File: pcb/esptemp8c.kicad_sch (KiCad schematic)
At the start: 19 parts, among them J1 T1, J2 T2, J4 T3, J6 T4, SW1 RESET, U1 ESP32-C3-MINI-1

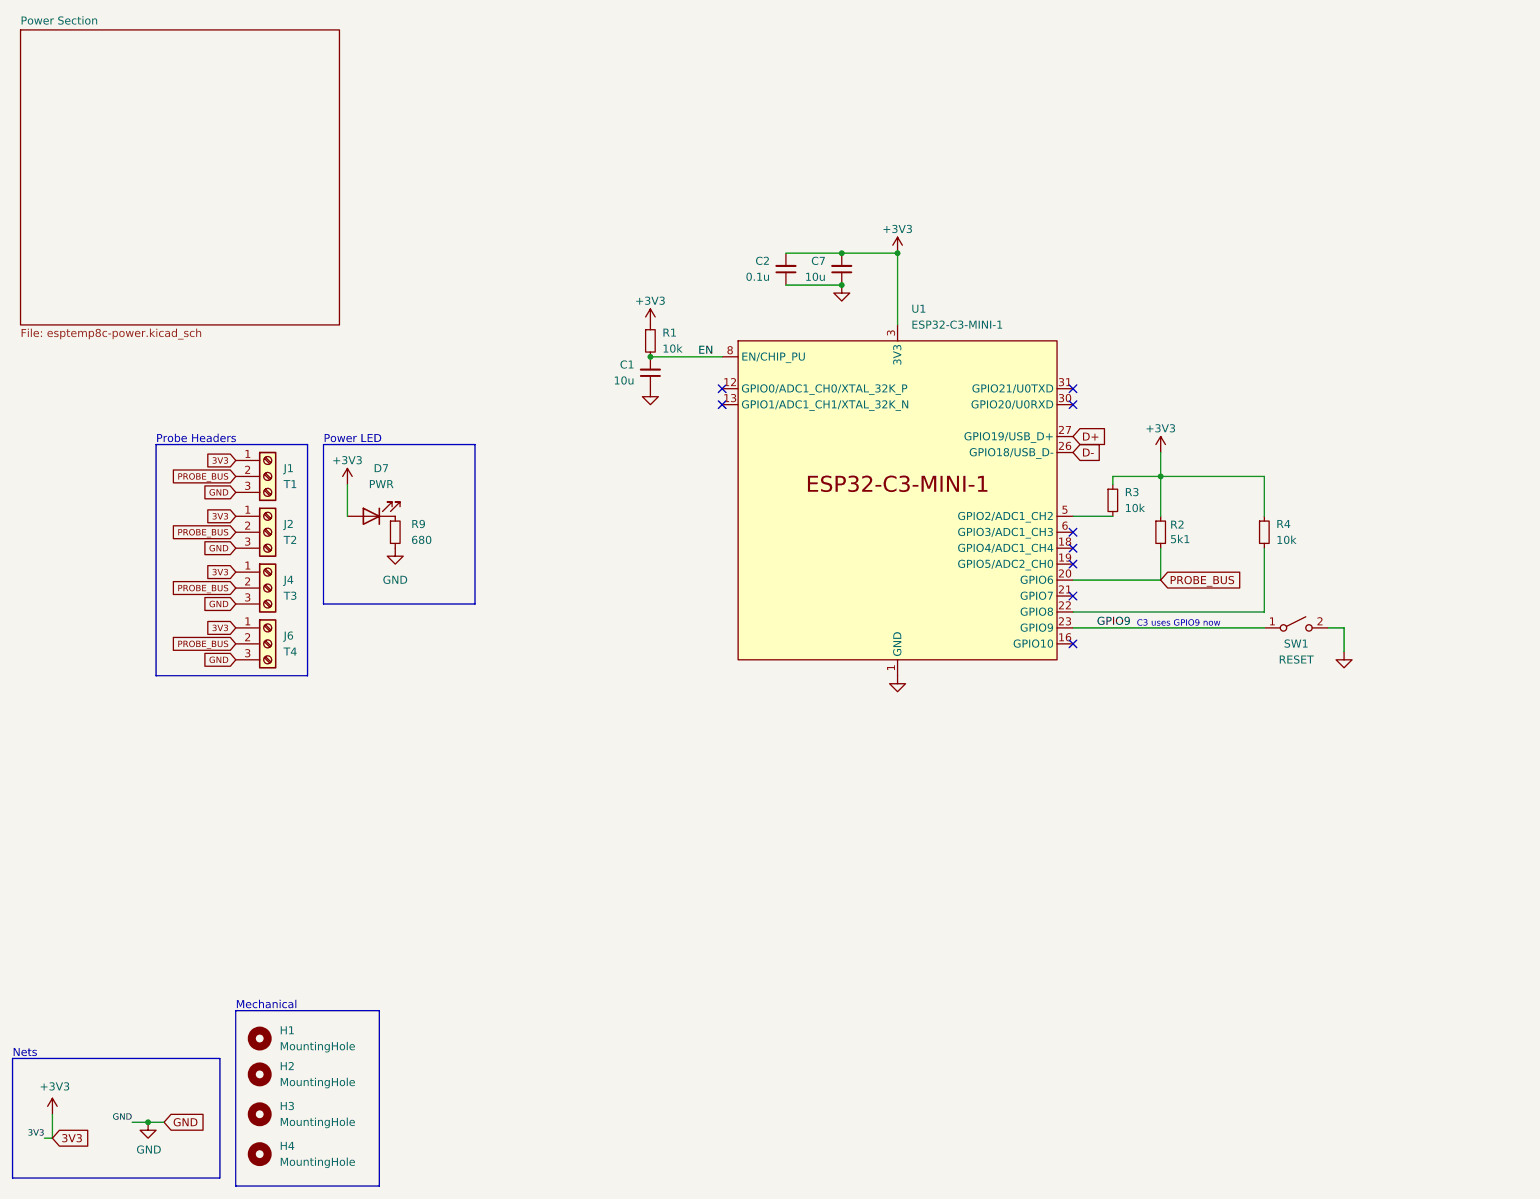
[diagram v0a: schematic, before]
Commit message: final touches and check
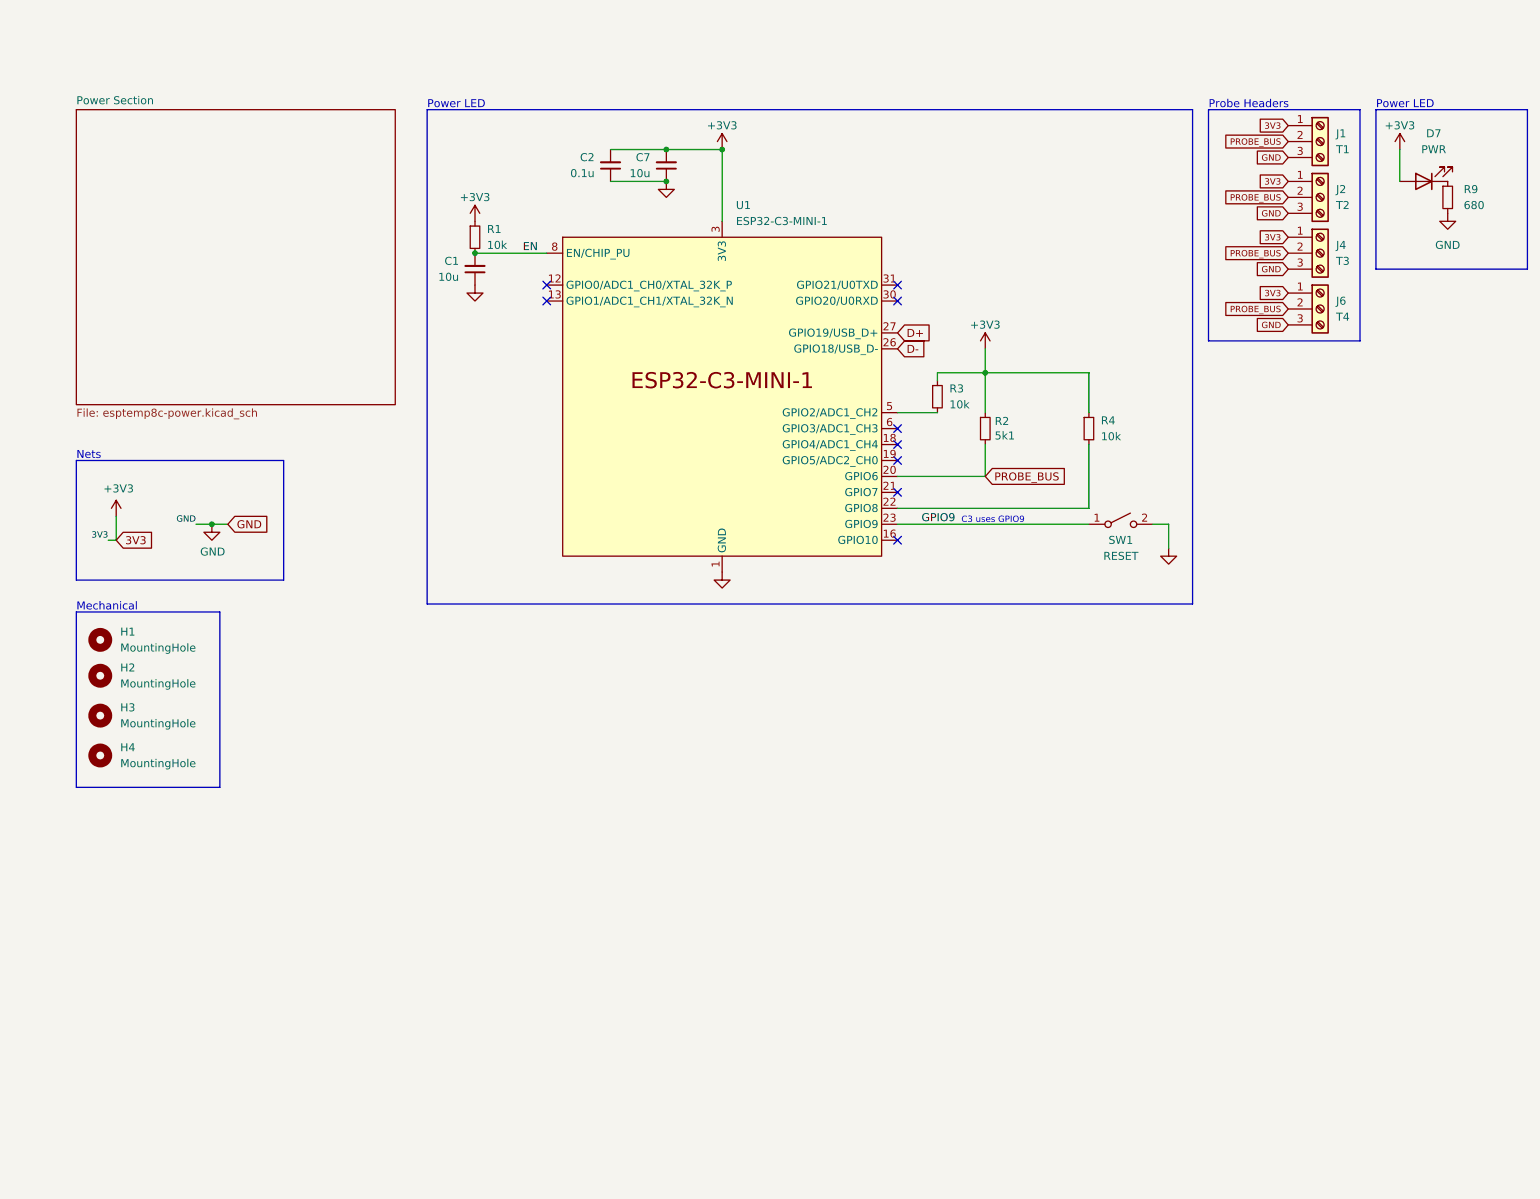
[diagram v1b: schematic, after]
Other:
- note added: "C3 uses GPIO9"
- note removed: "C3 uses GPIO9 now"
- moved on the sheet: C1, C2, C7, D7, H1, H2, H3, H4, J1, J2, J4, J6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

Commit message: panel touchup, alternate pn
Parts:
- J1, J2, J6: LCSC Alt (none) -> C5188158
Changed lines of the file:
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@@
+			)
+		)
+		(property "LCSC Alt" "C5188158"
+			(at 222.25 34.29 0)
+			(effects
+				(font
+					(size 1.27 1.27)
+				)
+				(hide yes)
 			)
 		)
@@
 			)
 		)
+		(property "LCSC Alt" "C5188158"
+			(at 222.25 43.18 0)
+			(effects
+				(font
+					(size 1.27 1.27)
+				)
+				(hide yes)
+			)
+		)
 		(pin "1"
 		)
@@
 			(at 222.25 60.96 0)
 			(effects
+				(font
+					(size 1.27 1.27)
+				)
+				(hide yes)
+			)
+		)
+		(property "LCSC Alt" "C5188158"
+			(at 222.25 60.96 0)
+			(effects
